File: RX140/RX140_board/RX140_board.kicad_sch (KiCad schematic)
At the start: 1 part, among them U1 RX140

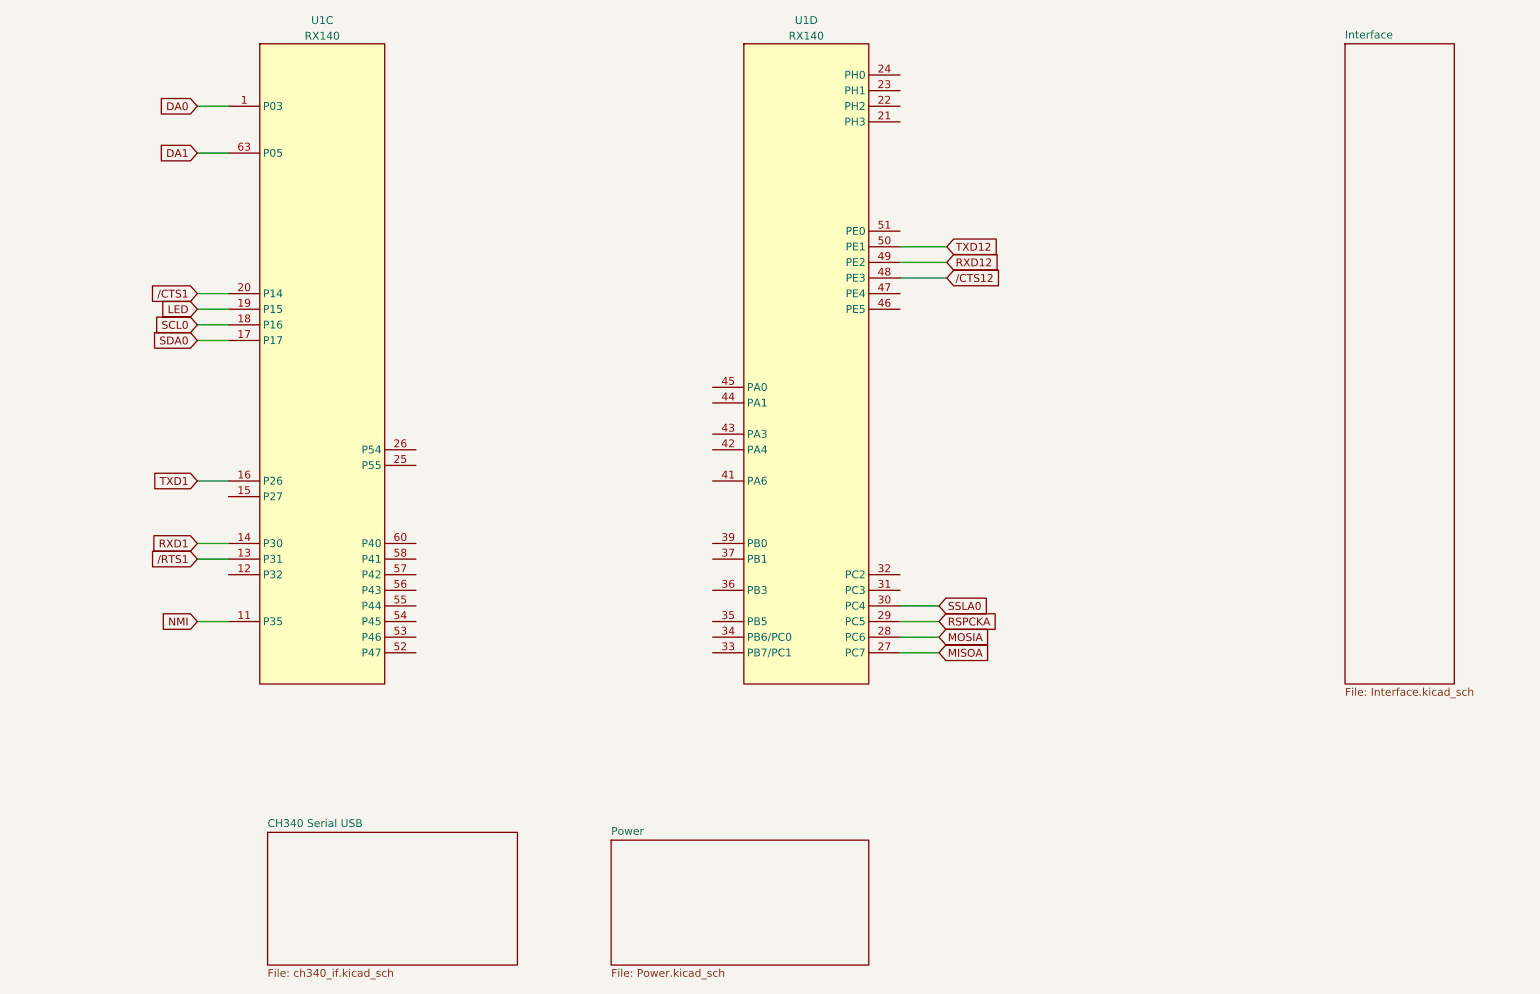
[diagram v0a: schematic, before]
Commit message: Update: cleanup
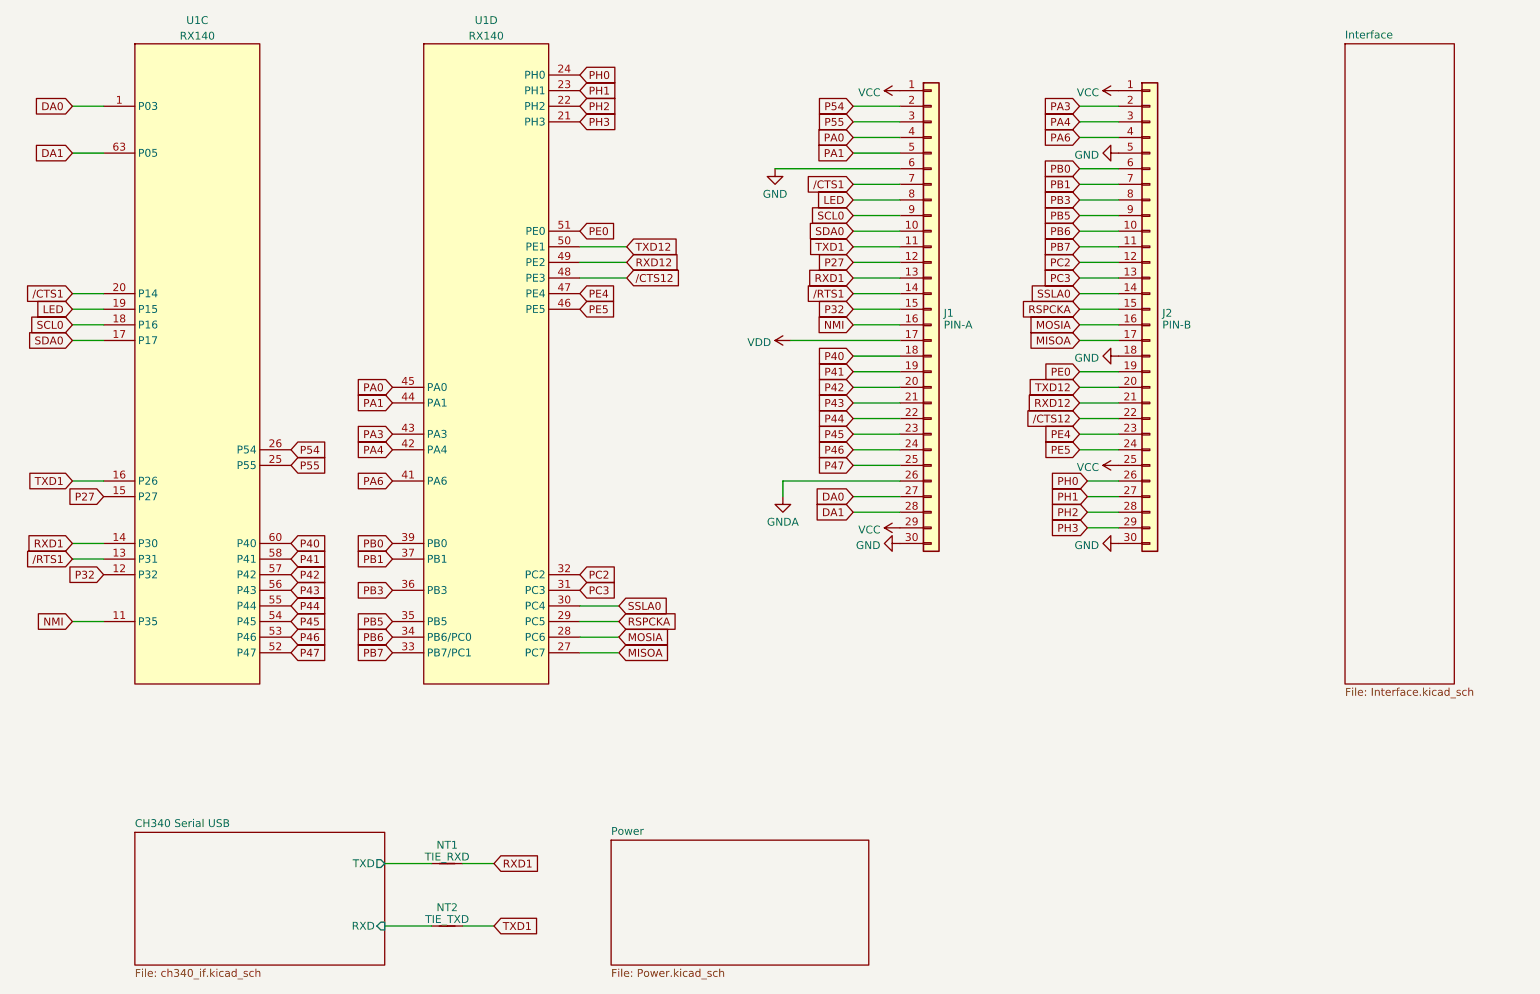
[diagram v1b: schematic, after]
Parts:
- added J1: PIN-A, Connector_PinHeader_2.54mm:PinHeader_1x30_P2.54mm_Vertical, symbol Connector_Generic:Conn_01x30
- added J2: PIN-B, Connector_PinHeader_2.54mm:PinHeader_1x30_P2.54mm_Vertical, symbol Connector_Generic:Conn_01x30
- added NT1: TIE_RXD, Connector_PinHeader_2.54mm:PinHeader_1x02_P2.54mm_Vertical, symbol Device:NetTie_2
- added NT2: TIE_TXD, Connector_PinHeader_2.54mm:PinHeader_1x02_P2.54mm_Vertical, symbol Device:NetTie_2
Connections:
- net DA0: now also J1.27 (Pin_27)
- net DA1: now also J1.28 (Pin_28)
- net LED: now also J1.8 (Pin_8)
- net MISOA: now also J2.17 (Pin_17)
- net MOSIA: now also J2.16 (Pin_16)
- net NMI: now also J1.16 (Pin_16)
- net RSPCKA: now also J2.15 (Pin_15)
- net RXD1: now also J1.13 (Pin_13), NT1.2
- net RXD12: now also J2.21 (Pin_21)
- net SCL0: now also J1.9 (Pin_9)
- net SDA0: now also J1.10 (Pin_10)
- net SSLA0: now also J2.14 (Pin_14)
- net TXD1: now also J1.11 (Pin_11), NT2.2
- net TXD12: now also J2.20 (Pin_20)
- net /CTS1: now also J1.7 (Pin_7)
- net /CTS12: now also J2.22 (Pin_22)
- net /RTS1: now also J1.14 (Pin_14)
- net P32: now reaches U1.12 (P32)
- net P32: now also J1.15 (Pin_15)
- net P27: now reaches U1.15 (P27)
- net P27: now also J1.12 (Pin_12)
- net P55: now reaches U1.25 (P55)
- net P55: now also J1.3 (Pin_3)
- net P54: now reaches U1.26 (P54)
- net P54: now also J1.2 (Pin_2)
- net P47: now reaches U1.52 (P47)
- net P47: now also J1.25 (Pin_25)
- net P46: now reaches U1.53 (P46)
- net P46: now also J1.24 (Pin_24)
- net P45: now reaches U1.54 (P45)
- net P45: now also J1.23 (Pin_23)
- net P44: now reaches U1.55 (P44)
- net P44: now also J1.22 (Pin_22)
- net P43: now reaches U1.56 (P43)
- net P43: now also J1.21 (Pin_21)
- net P42: now reaches U1.57 (P42)
- net P42: now also J1.20 (Pin_20)
- net P41: now reaches U1.58 (P41)
- net P41: now also J1.19 (Pin_19)
- net P40: now reaches U1.60 (P40)
- net P40: now also J1.18 (Pin_18)
- net PH3: now reaches U1.21 (PH3)
- net PH3: now also J2.29 (Pin_29)
- net PH2: now reaches U1.22 (PH2)
- net PH2: now also J2.28 (Pin_28)
- net PH1: now reaches U1.23 (PH1)
- net PH1: now also J2.27 (Pin_27)
- net PH0: now reaches U1.24 (PH0)
- net PH0: now also J2.26 (Pin_26)
- net PC3: now reaches U1.31 (PC3)
- net PC3: now also J2.13 (Pin_13)
- net PC2: now reaches U1.32 (PC2)
- net PC2: now also J2.12 (Pin_12)
- net PB7: now reaches U1.33 (PB7/PC1)
- net PB7: now also J2.11 (Pin_11)
- net PB6: now reaches U1.34 (PB6/PC0)
- net PB6: now also J2.10 (Pin_10)
- net PB5: now reaches U1.35 (PB5)
- net PB5: now also J2.9 (Pin_9)
- net PB3: now reaches U1.36 (PB3)
- net PB3: now also J2.8 (Pin_8)
- net PB1: now reaches U1.37 (PB1)
- net PB1: now also J2.7 (Pin_7)
- net PB0: now reaches U1.39 (PB0)
- net PB0: now also J2.6 (Pin_6)
- net PA6: now reaches U1.41 (PA6)
- net PA6: now also J2.4 (Pin_4)
- net PA4: now reaches U1.42 (PA4)
- net PA4: now also J2.3 (Pin_3)
- net PA3: now reaches U1.43 (PA3)
- net PA3: now also J2.2 (Pin_2)
- net PA1: now reaches U1.44 (PA1)
- net PA1: now also J1.5 (Pin_5)
- net PA0: now reaches U1.45 (PA0)
- net PA0: now also J1.4 (Pin_4)
- net PE5: now reaches U1.46 (PE5)
- net PE5: now also J2.24 (Pin_24)
- net PE4: now reaches U1.47 (PE4)
- net PE4: now also J2.23 (Pin_23)
- net PE0: now reaches U1.51 (PE0)
- net PE0: now also J2.19 (Pin_19)
- new net CH340 Serial USB/RXD: NT2.1
- new net CH340 Serial USB/TXD: NT1.1
- new net GND: J1.30 (Pin_30), J1.6 (Pin_6), J2.18 (Pin_18), J2.30 (Pin_30), J2.5 (Pin_5)
- new net GNDA: J1.26 (Pin_26)
- new net VCC: J1.1 (Pin_1), J1.29 (Pin_29), J2.1 (Pin_1), J2.25 (Pin_25)
- new net VDD: J1.17 (Pin_17)
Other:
- sheet CH340 Serial USB ports: added RXD, TXD; removed none
- moved on the sheet: U1C, U1D
